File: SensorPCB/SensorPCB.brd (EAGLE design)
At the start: 35.2 x 66 mm, 31 parts, among them T1 33u

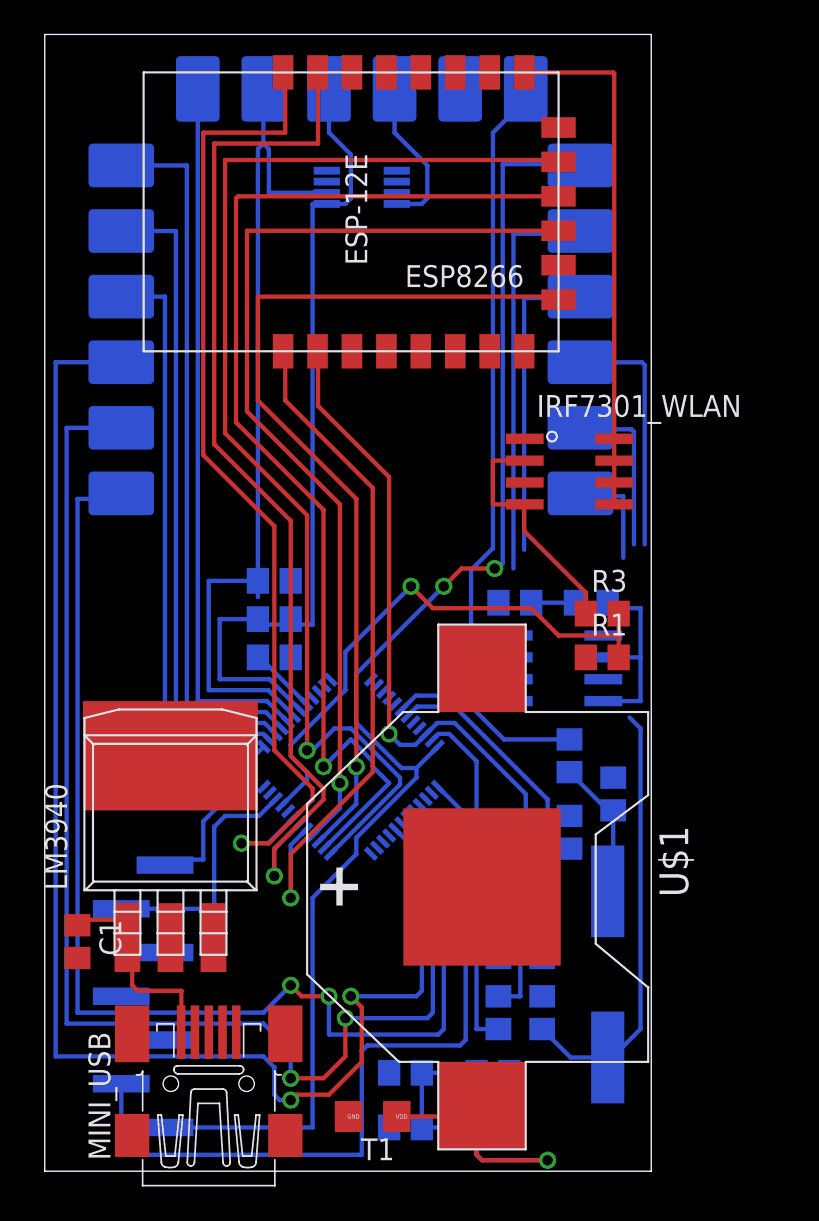
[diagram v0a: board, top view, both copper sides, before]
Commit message: layout update
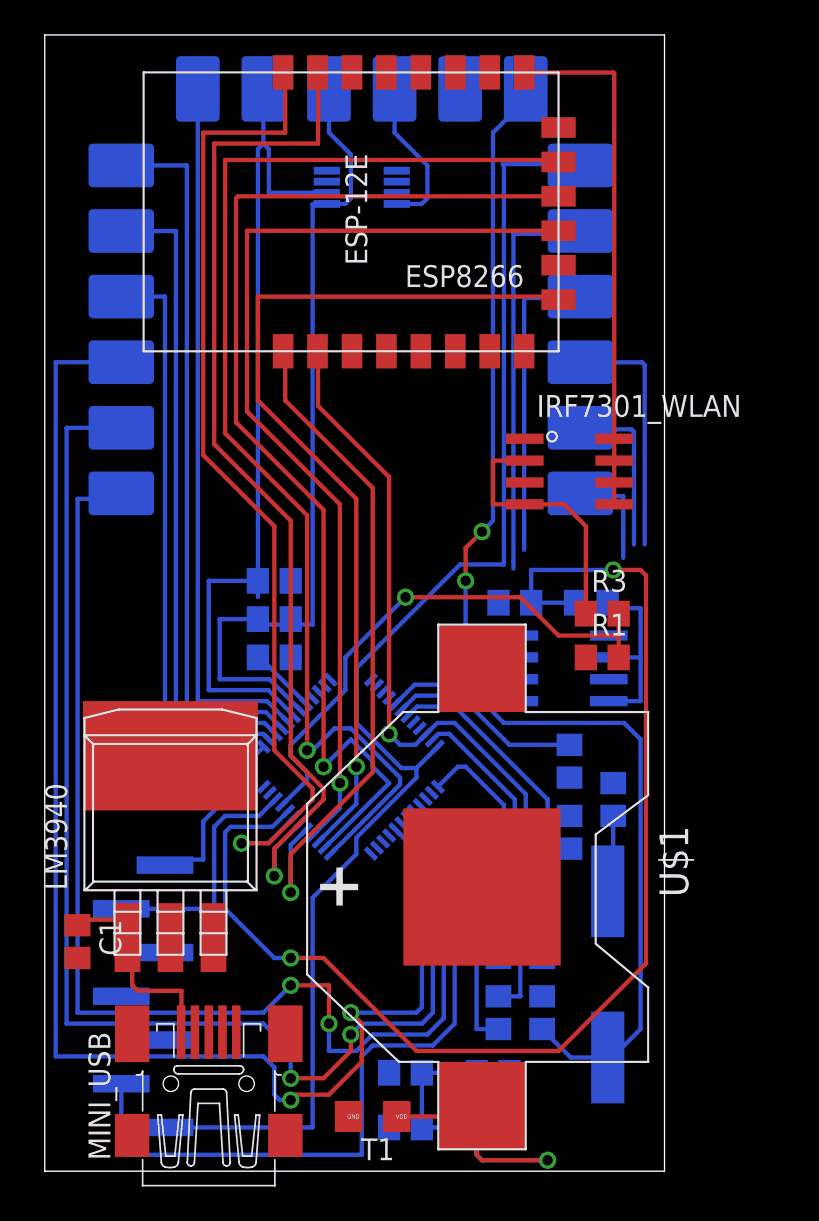
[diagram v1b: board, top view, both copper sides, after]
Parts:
- moved IRF7301_SENSOR 0.32 mm to (30.2, 29.2)
- moved C6 0.32 mm to (33.0, 21.6)
- moved R11 0.32 mm to (30.5, 23.8)
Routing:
- net SW_SENSOR: track 2.55 -> 72.4 mm, vias 0 -> 2
- net OSC_IN: track 25.4 -> 39.9 mm
- net USART2_RX_SENSOR: track 69.4 -> 73.6 mm
- net N$4: track 8.29 -> 4.96 mm
- net N$1: track 20.2 -> 23.0 mm
- net GATE_WLAN: track 14.5 -> 15.8 mm
- net PB0: track 70.2 -> 71.6 mm
- net GND_SENSOR: track 39.0 -> 39.7 mm, vias 0 -> 2
- net PB1: track 75.9 -> 75.2 mm
- net SW_WLAN: track 32.4 -> 31.7 mm
- net GATE_SENSOR: track 11.8 -> 11.1 mm
- net REST_WLAN: track 40.2 -> 39.6 mm
- net USART2_TX_SENSOR: vias 2 -> 0
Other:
- board size 35.2 x 66 mm -> 36 x 66 mm
